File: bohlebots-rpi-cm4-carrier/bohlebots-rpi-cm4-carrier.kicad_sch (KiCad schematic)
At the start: 30 parts, among them J1 SI-46001-F, J2 power_reference, J3 IO_Conn_02x05, J4 I2C_Conn_1x04, K1 Kicker, T1 Taster_LED, T2 Taster_LED, U1 Compute_Module_4_Connectors, U2 USB_Conn_01x05_Pin, U3 DT1446-04SO-7, U5 DT1446-04SO-7, X1 Miromatch

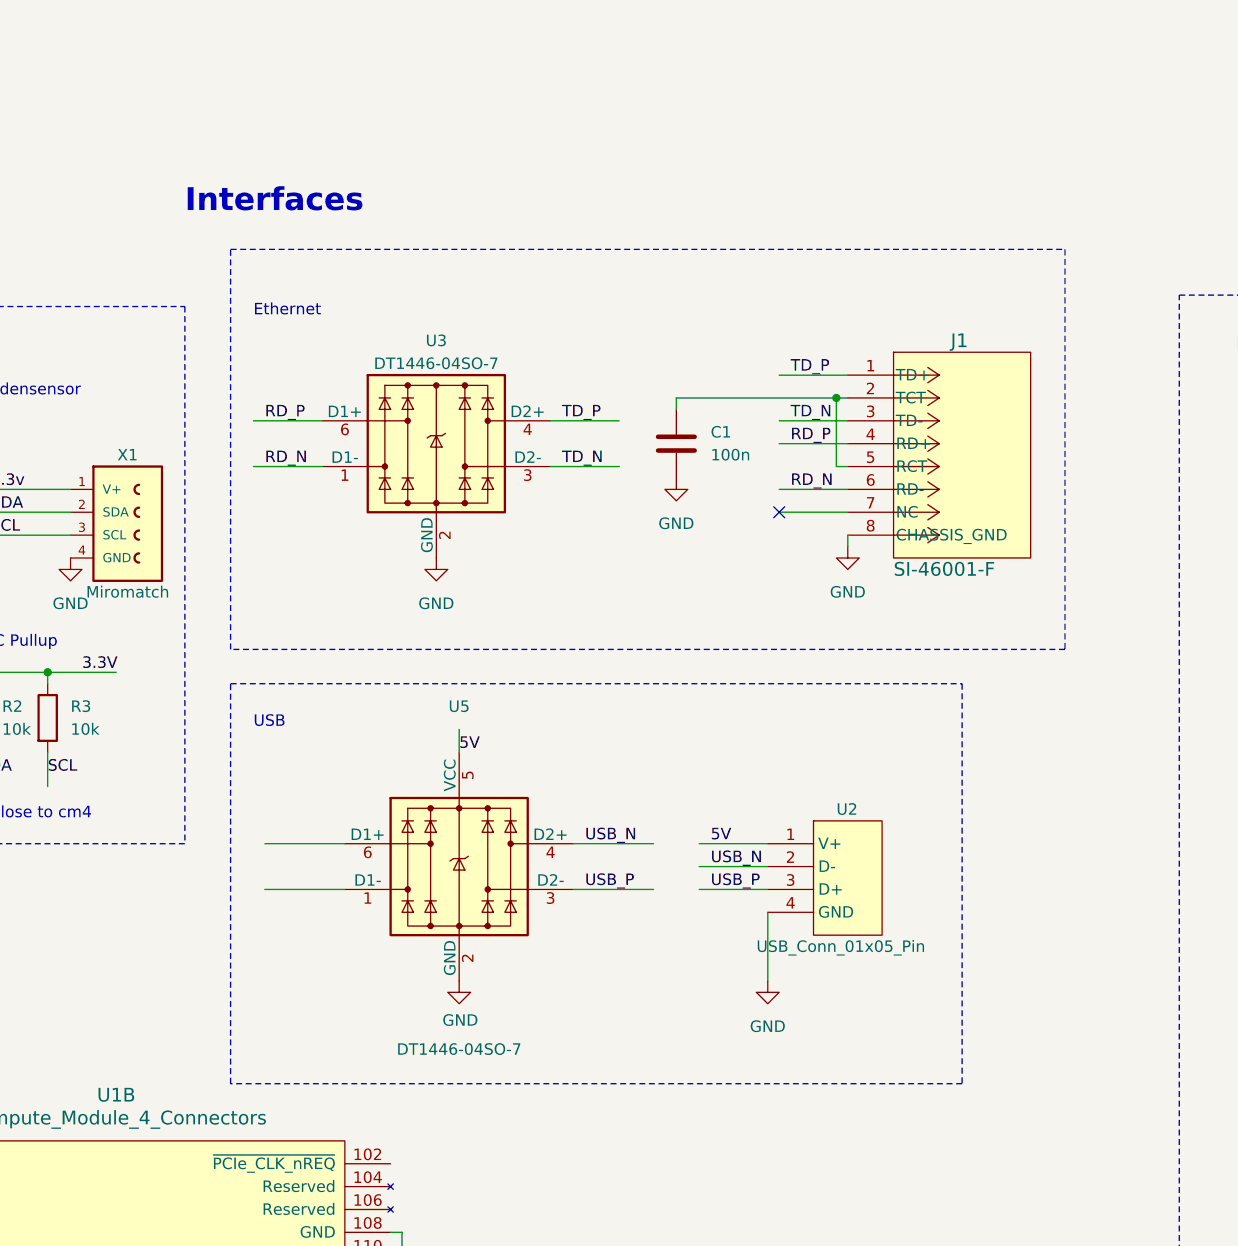
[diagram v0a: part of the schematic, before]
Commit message: Started routing.
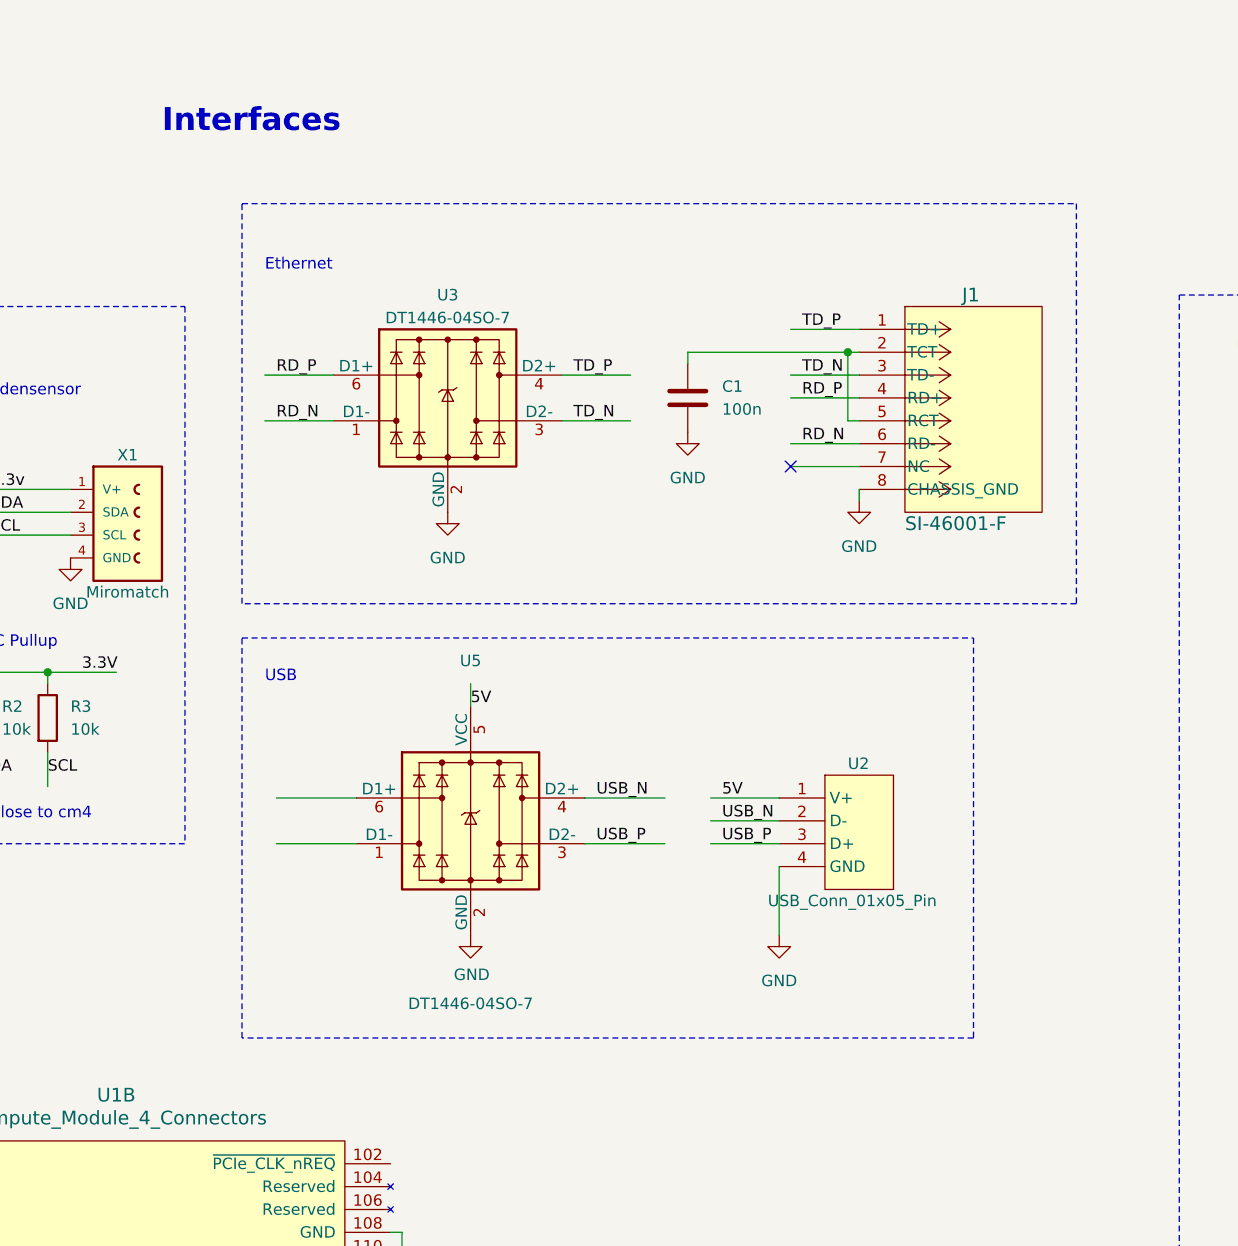
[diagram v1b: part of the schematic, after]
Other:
- moved on the sheet: C1, J1, U2, U3, U5
